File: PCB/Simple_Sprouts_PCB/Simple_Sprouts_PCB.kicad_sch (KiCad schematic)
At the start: 45 parts, among them J1 Raspberry_Pi_5, J10 NoIR Camera Module, J11 Fan, J3 Soil Sensor, J4 Soil Sensor, J6 Temperature Sensor, J7 Air Quality Sensor, J8 Humidity Sensor, J9 HC-SR04, Q1 IRLB8721PbF, Q2 IRLB8721PbF, Q3 IRLB8721PbF, Q4 IRLB8721PbF, Q5 IRLB8721PbF, Q6 IRLB8721PbF, U1 DC-DC Converter, U2 DC-DC Converter

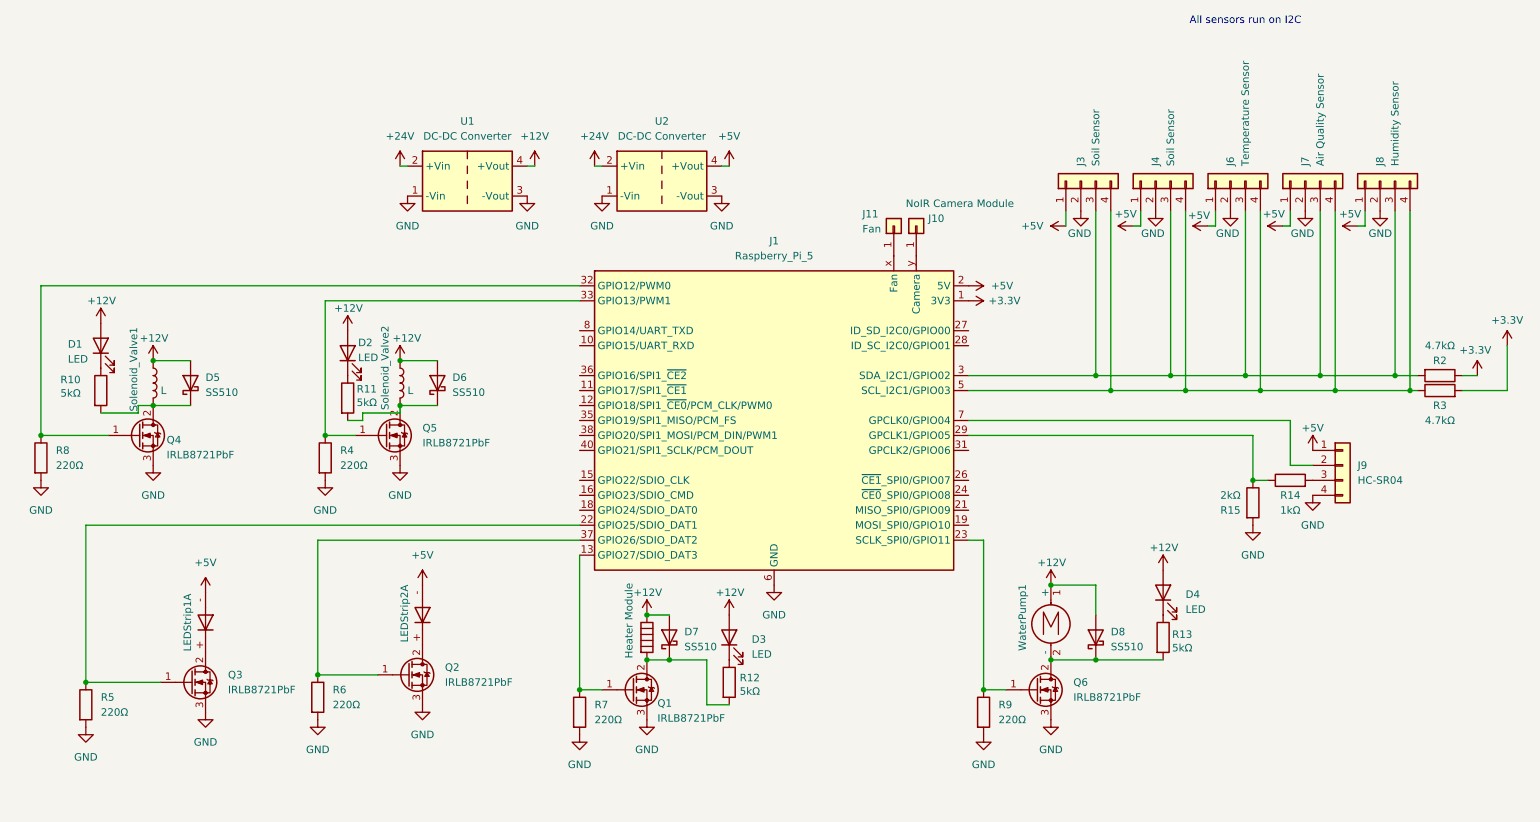
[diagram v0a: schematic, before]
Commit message: Add files via upload
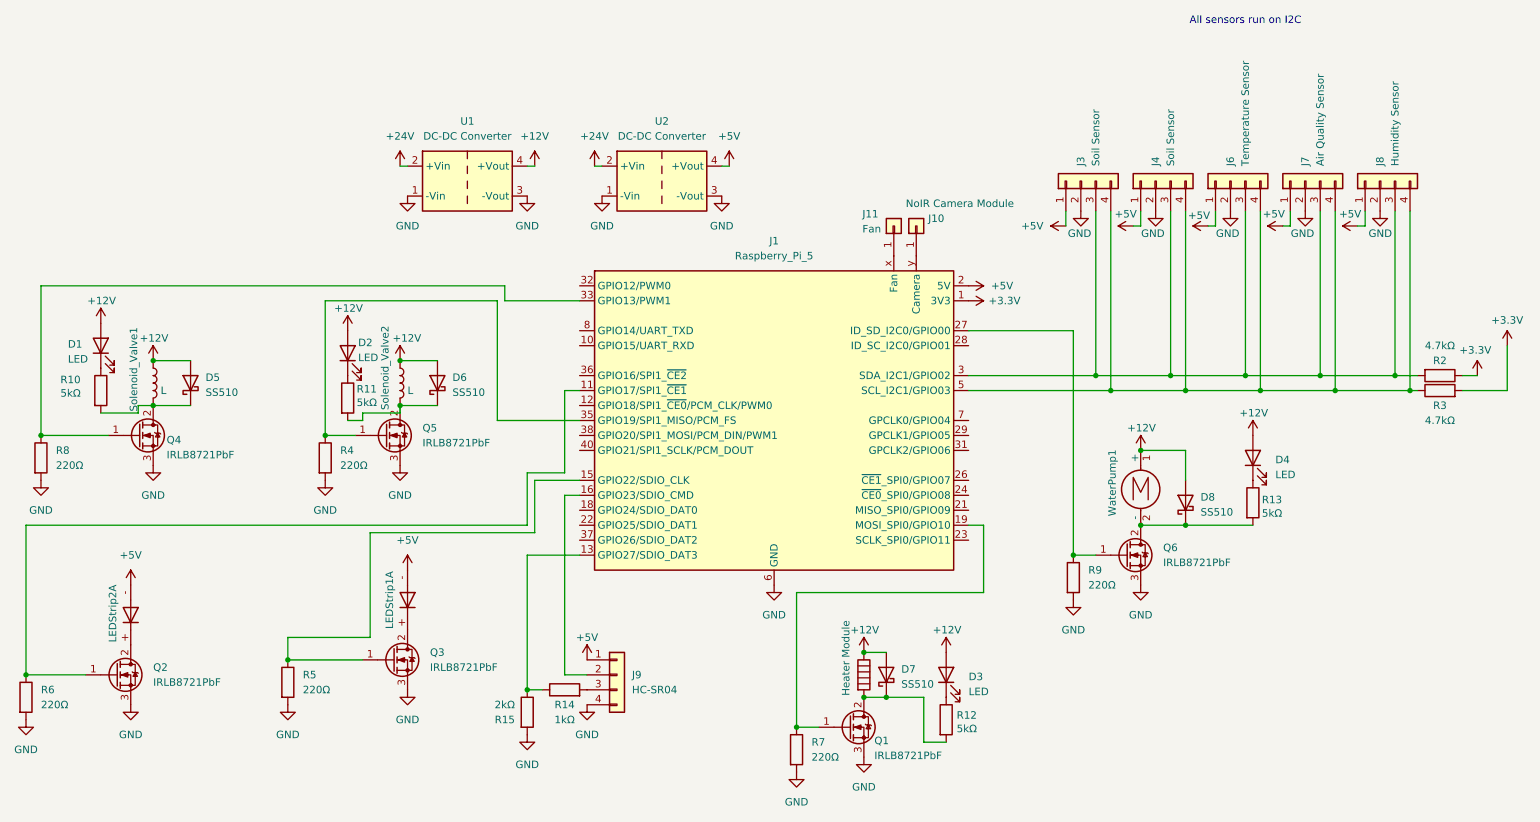
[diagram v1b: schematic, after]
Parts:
- J1: footprint RASPBERRY_PI_4B_4GB:MODULE_RASPBERRY_PI_4B_4GB -> RASPBERRY_PI_4B_4GB:Pin_Replacement
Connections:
- net at Q1.1 (G), R7.1: now also J1.19 (MOSI_SPI0/GPIO10); no longer J1.13 (GPIO27/SDIO_DAT3)
- net at Q6.1 (G), R9.1: now also J1.27 (ID_SD_I2C0/GPIO00); no longer J1.23 (SCLK_SPI0/GPIO11)
- net at Q4.1 (G), R8.1: now also J1.33 (GPIO13/PWM1); no longer J1.32 (GPIO12/PWM0)
- net at R14.1, R15.1: now also J1.13 (GPIO27/SDIO_DAT3); no longer J1.29 (GPCLK1/GPIO05)
- net at Q2.1 (G), R6.1: now also J1.11 (GPIO17/SPI1_~{CE1}); no longer J1.37 (GPIO26/SDIO_DAT2)
- net at Q5.1 (G), R4.1: now also J1.35 (GPIO19/SPI1_MISO/PCM_FS); no longer J1.33 (GPIO13/PWM1)
- net at J1.15 (GPIO22/SDIO_CLK): now also Q3.1 (G), R5.1
- net at J1.16 (GPIO23/SDIO_CMD): now also J9.2 (Pin_2)
- net at J1.7 (GPCLK0/GPIO04): no longer J9.2 (Pin_2)
- now unconnected: J1.22 (GPIO25/SDIO_DAT1)
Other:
- moved on the sheet: D3, D4, D7, D8, J9, LEDStrip1A, LEDStrip2A, Q1, Q2, Q3, Q6, R12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
